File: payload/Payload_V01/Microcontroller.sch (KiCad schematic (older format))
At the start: 1 part, among them U4 STM32F407VETx

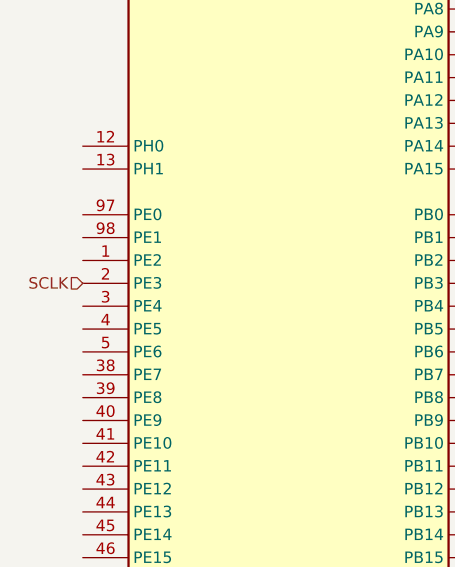
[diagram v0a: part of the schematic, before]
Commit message: small change
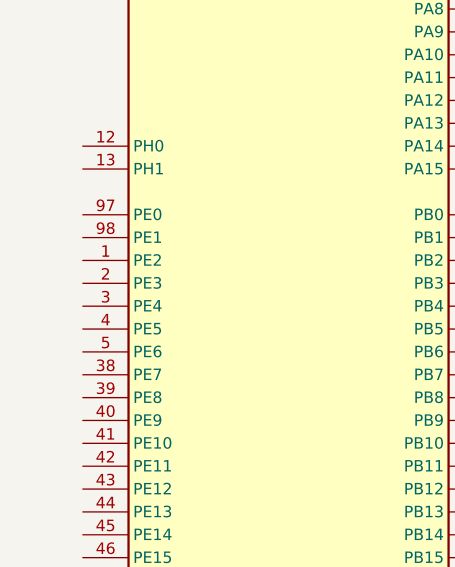
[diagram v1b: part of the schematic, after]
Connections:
- net SCLK: no longer names the net of U4.2 (PE3)
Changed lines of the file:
@@
 	1    0    0    -1
 $EndComp
-Text HLabel 4450 3450 0    50   Input ~ 0
-SCLK
 $EndSCHEMATC
